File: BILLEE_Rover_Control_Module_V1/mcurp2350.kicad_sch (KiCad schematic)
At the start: 54 parts, among them CN6 DF11-18DP-2DSA, J1 2.54mm Header, SW2 KMR2, SW3 RESET SW, U10 RP2350A_C42411118, U11 ABM8-272-T3_C20625731, U12 W25Q128JVSIQTR, U13 TCA4307DGKR, U14 TCA4307DGKR, U15 TXS0108EPWR

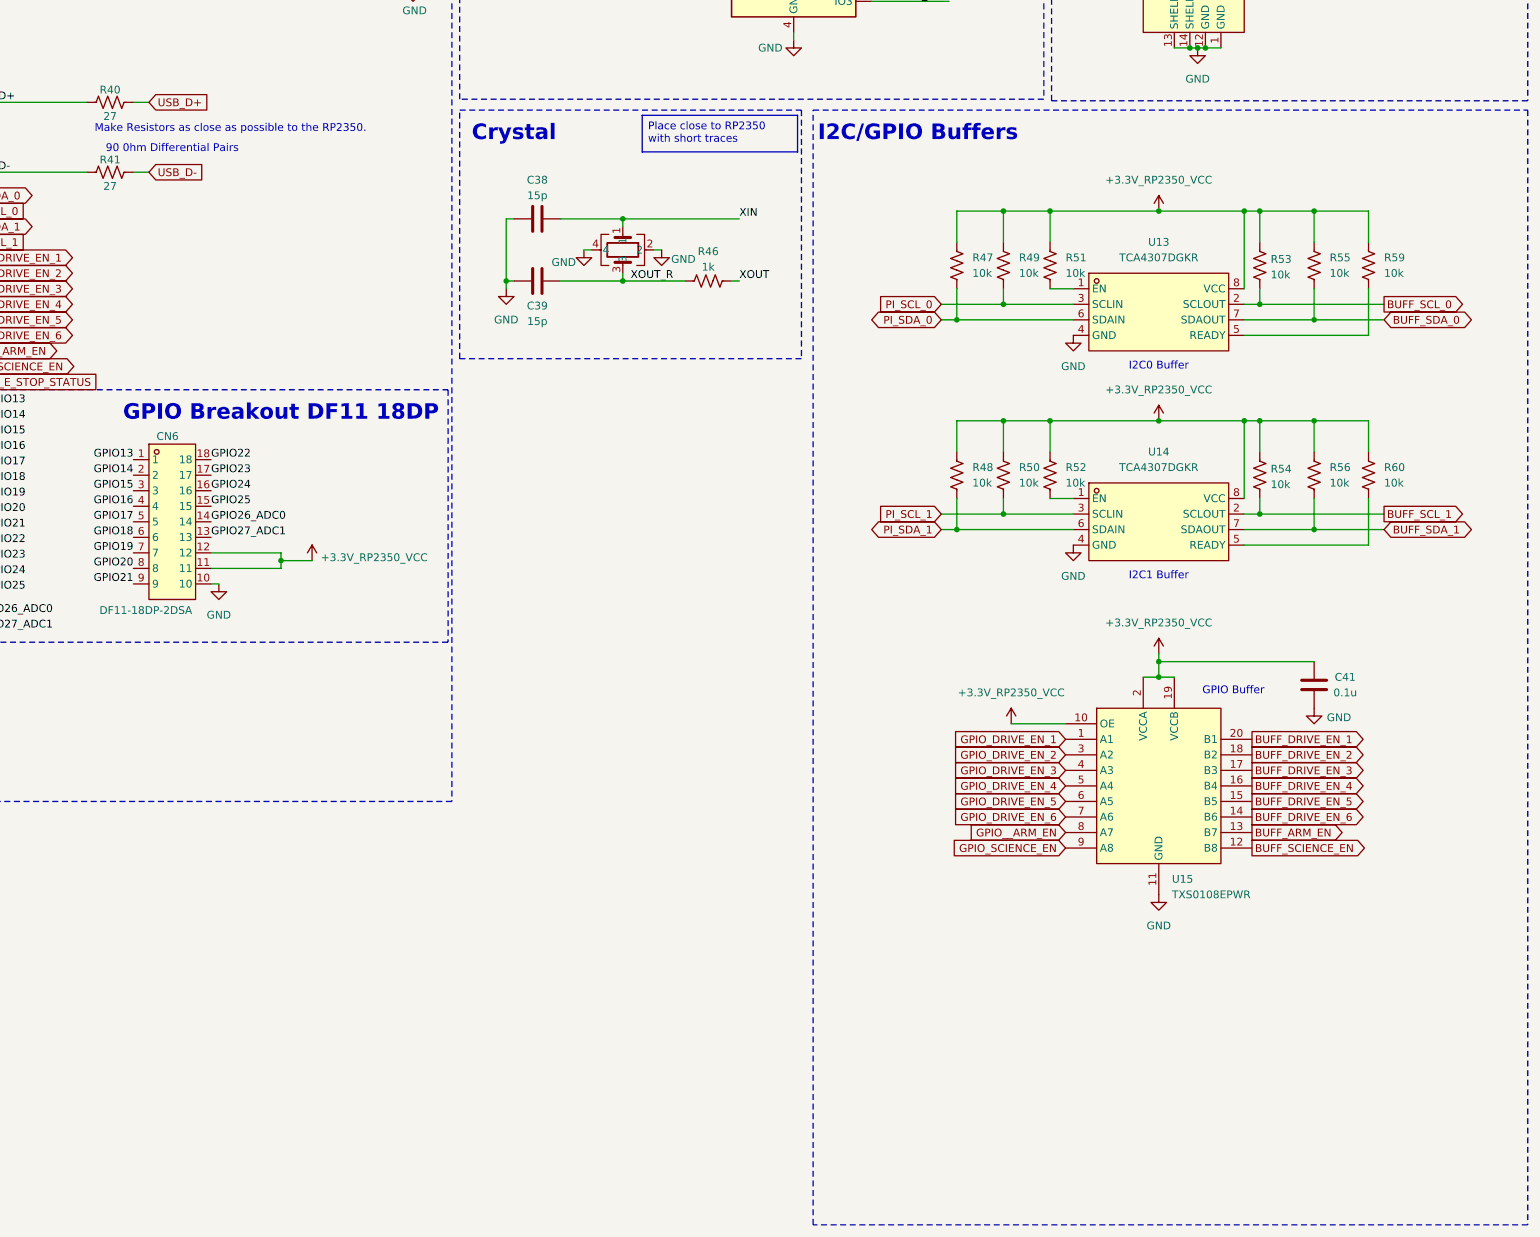
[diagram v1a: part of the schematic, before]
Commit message: More layout :tired_face:
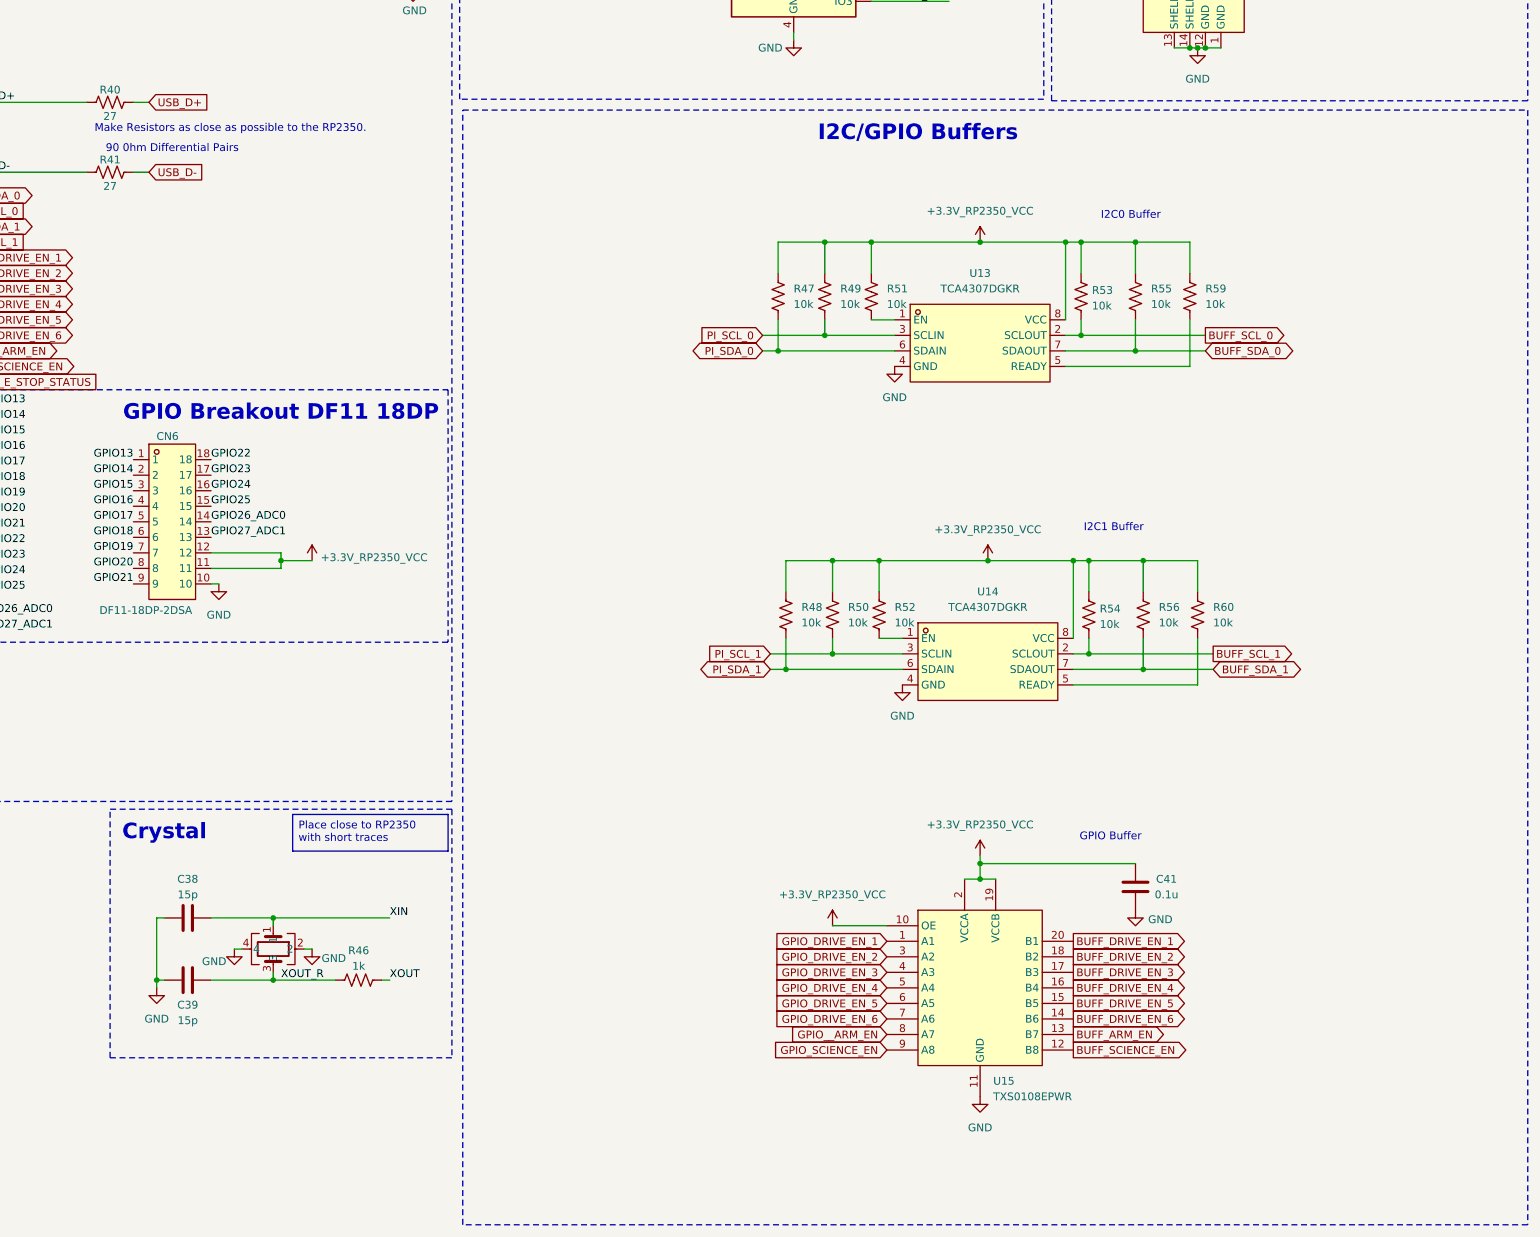
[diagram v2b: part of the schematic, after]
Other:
- moved on the sheet: C38, C39, C41, R46, R47, R48, R49, R50, R51, R52, R53, R54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
